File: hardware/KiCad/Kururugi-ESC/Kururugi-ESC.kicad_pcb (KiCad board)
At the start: 6 copper layers, 37.9 x 23.6 mm, 141 parts, among them J1 Conn_01x01, J10 Conn_01x01, J11 Conn_01x01, J2 Conn_01x01, J3 Conn_01x01, J4 Conn_01x01, J5 Conn_01x01, J6 Conn_01x01, J7 Conn_01x01, J8 JTAG_TC2030, J9 Conn_01x01, Q1 CSD18540Q5B, Q2 CSD18540Q5B, Q3 CSD18540Q5B, Q4 CSD18540Q5B, Q5 CSD18540Q5B, Q6 CSD18540Q5B, U1 STM32G484CEU6, U2 LM5160A, U3 TPS7B92033, U4 2EDL8024, U5 2EDL8024, U6 2EDL8024, X1 16MHz

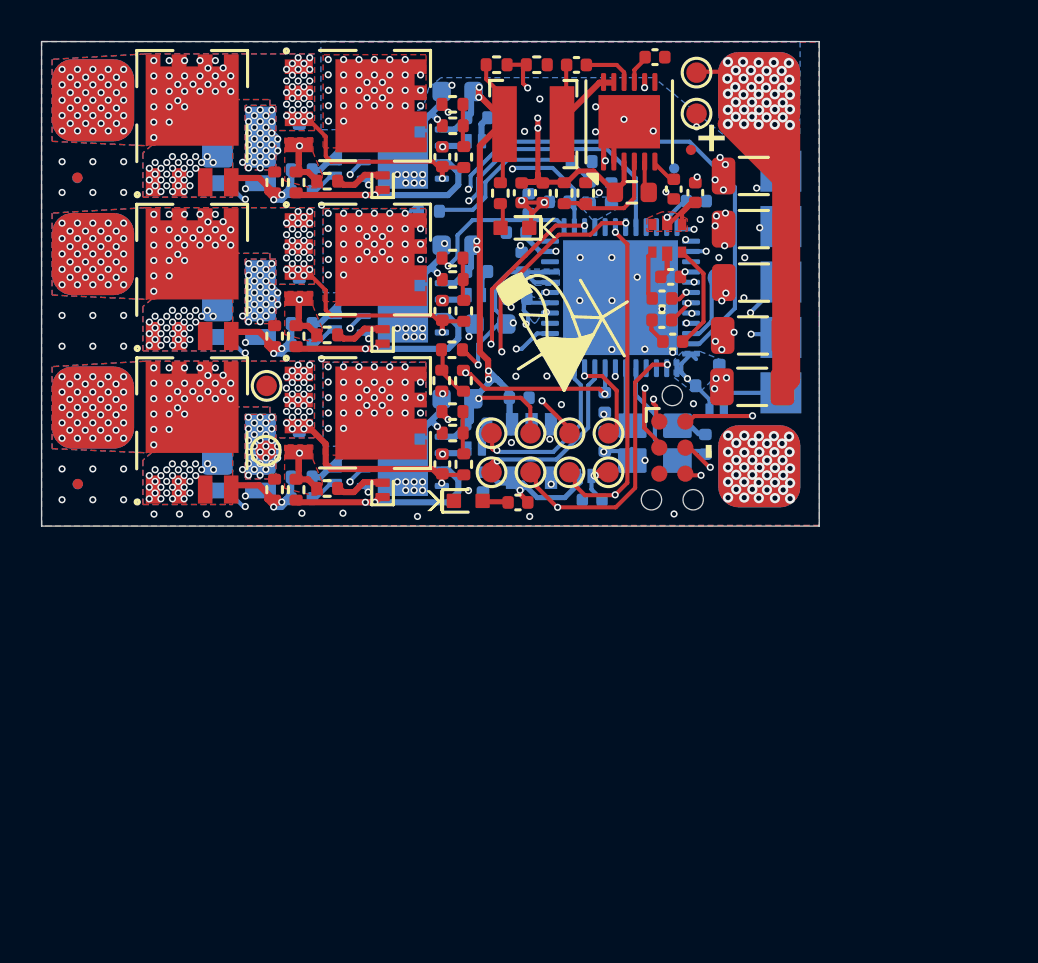
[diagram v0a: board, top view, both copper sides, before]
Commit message: Kicad minor corrections
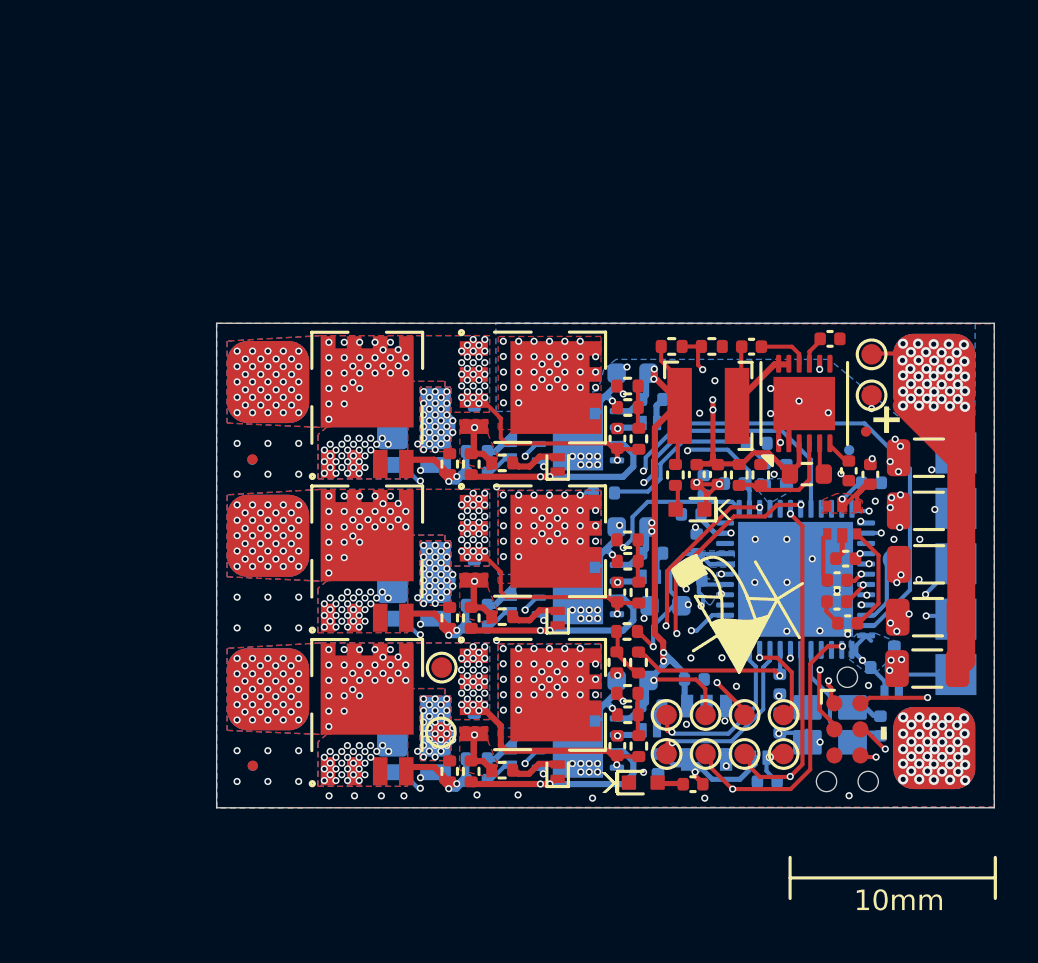
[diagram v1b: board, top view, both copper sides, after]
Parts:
- moved C10 16.2 mm to (112.8, 62.1)
- moved C11 16.2 mm to (113.9, 62.1)
- moved C14 16.2 mm to (120.2, 61.9)
- moved C16 16.2 mm to (112.8, 65.5)
- moved C25 16.2 mm to (109.0, 60.3)
- moved C28 16.2 mm to (109.0, 67.8)
- moved C3 16.2 mm to (124.2, 66.5)
- moved C32 16.2 mm to (109.7, 72.1)
- moved C6 16.2 mm to (117.2, 62.1)
- moved D11 16.2 mm to (110.5, 74.6)
- moved D12 16.2 mm to (106.1, 76.6)
- moved D3 16.2 mm to (115.9, 75.9)
- moved J9 16.2 mm to (91.9, 57.6)
- moved Q4 16.2 mm to (96.8, 66.3)
- moved R2 16.2 mm to (116.1, 62.1)
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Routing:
- net /TSENS: track 8.66 -> 8.58 mm, vias 2 -> 1
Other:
- rule pad_to_mask_clearance: 0 -> 0.05
- board text added: "10mm"
